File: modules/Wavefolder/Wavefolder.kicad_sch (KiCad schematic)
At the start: 16 parts, among them J10 Conn_Front, J104 WQP-PJ398, J105 WQP-PJ398, J106 WQP-PJ398, J107 WQP-PJ398, J11 Conn_Back, J9 Conn_Eurorack_10, U3 TL072

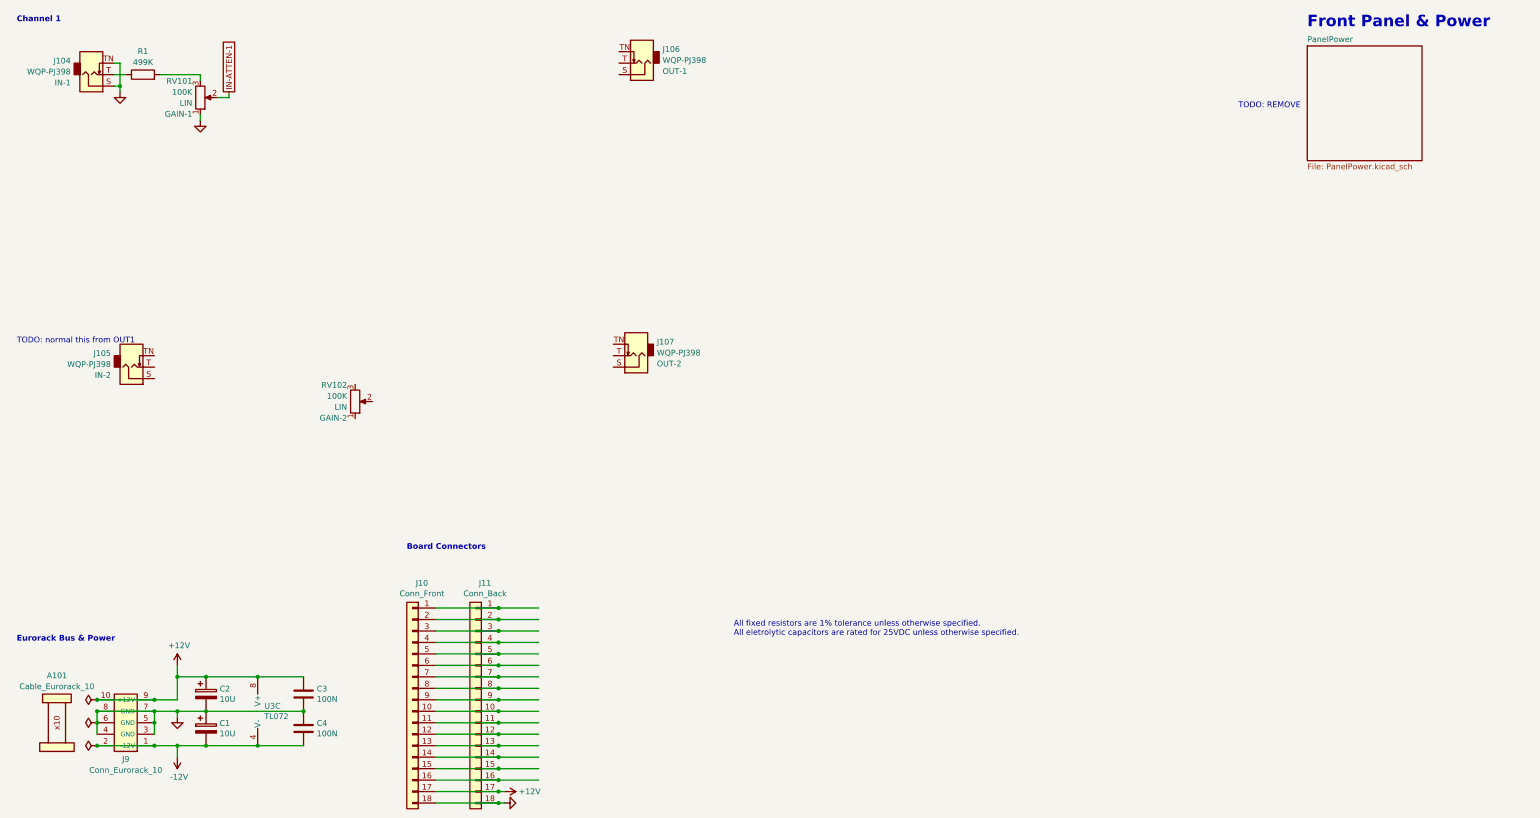
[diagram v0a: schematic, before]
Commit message: Munger re-design - schematic done, PCB started
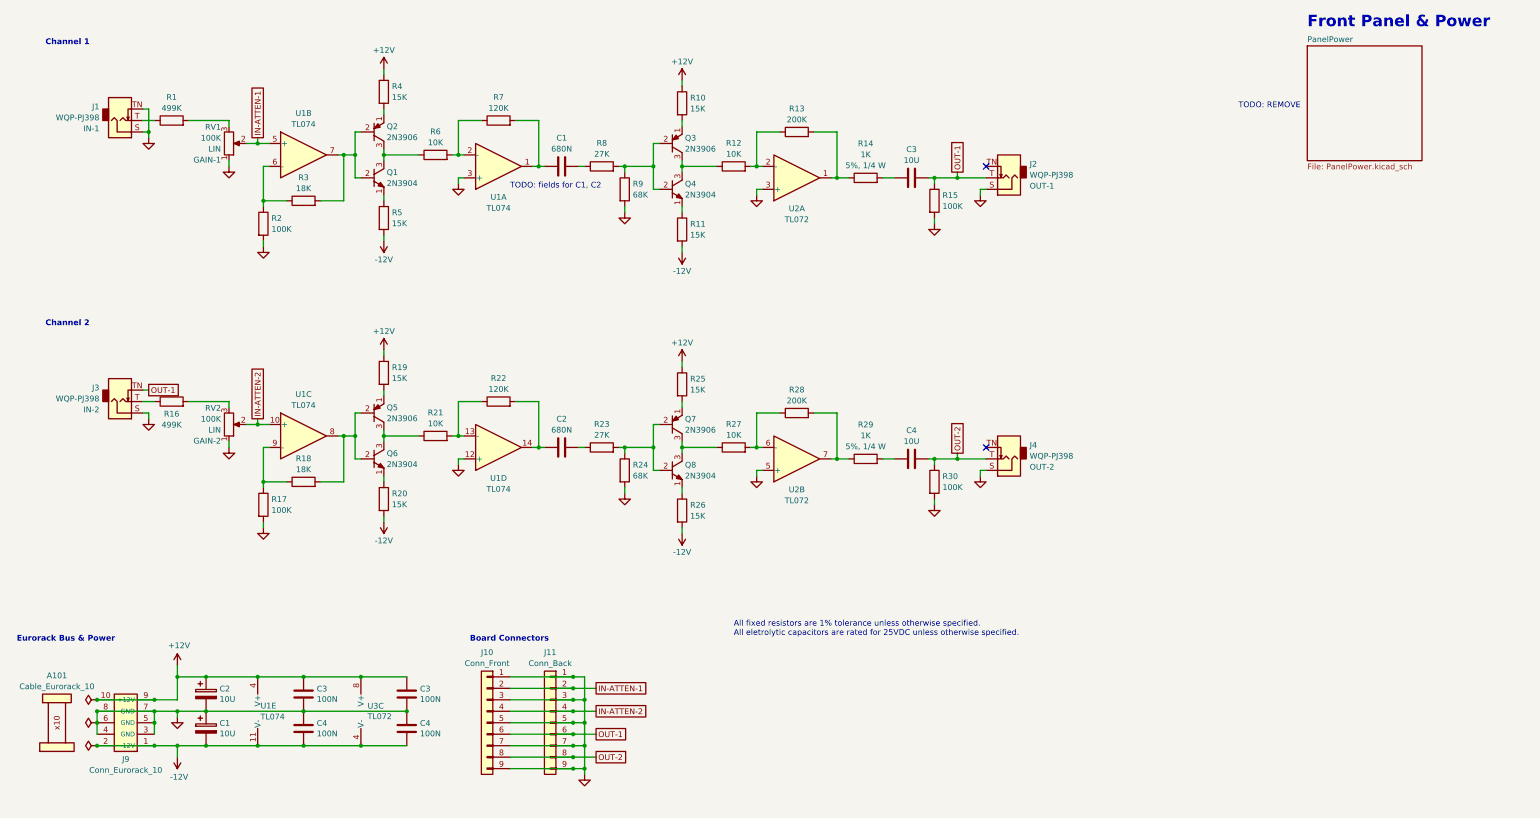
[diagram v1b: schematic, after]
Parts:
- added C1, C2: 680N, -lmp-misc:C_Rect_L7.2mm_W4.5mm_P5.00mm, symbol -lmp:CF
- added C3, C4: 10U, -lmp-misc:C_Radial_D5.0mm_H5.0mm_P2.50mm, symbol -lmp-synth:CNP_10U
- added C3, C4: 100N, -lmp-misc:C_Disc_D5.0mm_W2.5mm_P2.50mm, symbol -lmp:CC_100N
- added Q1, Q4, Q6, Q8: 2N3904, -lmp-misc:TO-92_Inline_Wide, symbol -lmp:Q_NPN_2N3904
- added Q2, Q3, Q5, Q7: 2N3906, -lmp-misc:TO-92_Inline_Wide, symbol -lmp:Q_PNP_2N3906
- added R10, R11, R19, R20, R25, R26, R4, R5: 15K, -lmp-misc:R_Axial_DIN0207_L6.3mm_D2.5mm_P7.62mm_Horizontal, symbol -lmp:R_1%_0W166
- added R12, R21, R27, R6: 10K, -lmp-misc:R_Axial_DIN0207_L6.3mm_D2.5mm_P7.62mm_Horizontal, symbol -lmp:R_1%_0W166
- added R13, R28: 200K, -lmp-misc:R_Axial_DIN0207_L6.3mm_D2.5mm_P7.62mm_Horizontal, symbol -lmp:R_1%_0W166
- added R14, R29: 1K, -lmp-misc:R_Axial_DIN0207_L6.3mm_D2.5mm_P10.16mm_Horizontal, symbol -lmp-synth:R_1K_Output
- added R15, R17, R2, R30: 100K, -lmp-misc:R_Axial_DIN0207_L6.3mm_D2.5mm_P7.62mm_Horizontal, symbol -lmp:R_1%_0W166
- added R16: 499K, -lmp-misc:R_Axial_DIN0207_L6.3mm_D2.5mm_P7.62mm_Horizontal, symbol -lmp:R_1%_0W166
- added R18, R3: 18K, -lmp-misc:R_Axial_DIN0207_L6.3mm_D2.5mm_P7.62mm_Horizontal, symbol -lmp:R_1%_0W166
- added R22, R7: 120K, -lmp-misc:R_Axial_DIN0207_L6.3mm_D2.5mm_P7.62mm_Horizontal, symbol -lmp:R_1%_0W166
- added R23, R8: 27K, -lmp-misc:R_Axial_DIN0207_L6.3mm_D2.5mm_P7.62mm_Horizontal, symbol -lmp:R_1%_0W166
- added R24, R9: 68K, -lmp-misc:R_Axial_DIN0207_L6.3mm_D2.5mm_P7.62mm_Horizontal, symbol -lmp:R_1%_0W166
- added U1: TL074, Package_DIP:DIP-14_W7.62mm, symbol -lmp-opamp:TL074
- added U2: TL072, Package_DIP:DIP-8_W7.62mm, symbol -lmp-opamp:TL072
- J10: footprint Connector_PinSocket_2.54mm:PinSocket_1x18_P2.54mm_Vertical -> Connector_PinSocket_2.54mm:PinSocket_1x09_P2.54mm_Vertical; symbol Connector_Generic:Conn_01x18 -> Connector_Generic:Conn_01x09
- J11: footprint Connector_PinHeader_2.54mm:PinHeader_1x18_P2.54mm_Horizontal -> Connector_PinHeader_2.54mm:PinHeader_1x09_P2.54mm_Horizontal; symbol Connector_Generic:Conn_01x18 -> Connector_Generic:Conn_01x09
- renumbered J104 to J1, J106 to J2, J105 to J3, J107 to J4, RV101 to RV1, RV102 to RV2
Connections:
- net +12V: now also C3.1, R10.1, R19.1, R25.1, R4.1, U1.4 (V+); no longer J10.17 (Pin_17), J11.17 (Pin_17)
- net -12V: now also C4.2, R11.2, R20.2, R26.2, R5.2, U1.11 (V-)
- net GND: now also J10.1 (Pin_1), J10.3 (Pin_3), J10.5 (Pin_5), J10.7 (Pin_7), J10.9 (Pin_9), J11.1 (Pin_1), J11.3 (Pin_3), J11.5 (Pin_5), J11.7 (Pin_7), J11.9 (Pin_9), J2.S, J3.S, J4.S, RV2.1, C3.2, C4.1, R15.2, R17.2, R2.2, R24.2, R30.2, R9.2, U1.12 (+), U1.3 (+), U2.3 (+), U2.5 (+); no longer J10.18 (Pin_18), J11.18 (Pin_18)
- net IN-ATTEN-1: now also J10.2 (Pin_2), J11.2 (Pin_2), U1.5 (+)
- net IN-ATTEN-2: now reaches J10.4 (Pin_4), J11.4 (Pin_4)
- net IN-ATTEN-2: now also RV2.2, U1.10 (+)
- net OUT-1: now reaches J10.6 (Pin_6), J11.6 (Pin_6)
- net OUT-1: now also J2.T, J3.TN, C3.2, R15.1
- net OUT-2: now reaches J10.8 (Pin_8), J11.8 (Pin_8)
- net OUT-2: now also J4.T, C4.2, R30.1
- net at RV2.3: now also R16.2
- net at J3.T: now also R16.1
- new net: Q6.1 (E), R20.1
- new net: C2.1, R22.2, U1.14
- new net: C2.2, R23.1
- new net: R13.2, R14.1, U2.1
- new net: R12.2, R13.1, U2.2 (-)
- new net: Q7.1 (E), R25.2
- new net: Q7.2 (B), Q8.2 (B), R23.2, R24.1
- new net: Q7.3 (C), Q8.3 (C), R27.1
- new net: Q5.2 (B), Q6.2 (B), R18.2, U1.8
- new net: R17.1, R18.1, U1.9 (-)
- new net: Q4.1 (E), R11.1
- new net: Q3.2 (B), Q4.2 (B), R8.2, R9.1
- new net: R2.1, R3.1, U1.6 (-)
- new net: Q1.2 (B), Q2.2 (B), R3.2, U1.7
- new net: C4.1, R29.2
- new net: Q3.1 (E), R10.2
- new net: R21.2, R22.1, U1.13 (-)
- new net: Q5.3 (C), Q6.3 (C), R21.1
- new net: Q2.1 (E), R4.2
- new net: C1.1, R7.2, U1.1
- new net: C1.2, R8.1
- new net: Q1.3 (C), Q2.3 (C), R6.1
- new net: R6.2, R7.1, U1.2 (-)
- new net: Q8.1 (E), R26.1
- new net: Q1.1 (E), R5.1
- new net: Q5.1 (E), R19.2
- new net: R27.2, R28.1, U2.6 (-)
- new net: C3.1, R14.2
- new net: Q3.3 (C), Q4.3 (C), R12.1
- new net: R28.2, R29.1, U2.7
- no-connect marks 0 -> 2
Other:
- note added: "Channel 2"
- note added: "TODO: fields for C1, C2"
- note removed: "TODO: normal this from OUT1"
- moved on the sheet: J1, J2, J3, J4, R1, RV1, RV2, U3C
